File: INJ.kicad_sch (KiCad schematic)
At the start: 10 parts, among them U2 VNLD5160TR-E, U3 VNLD5160TR-E

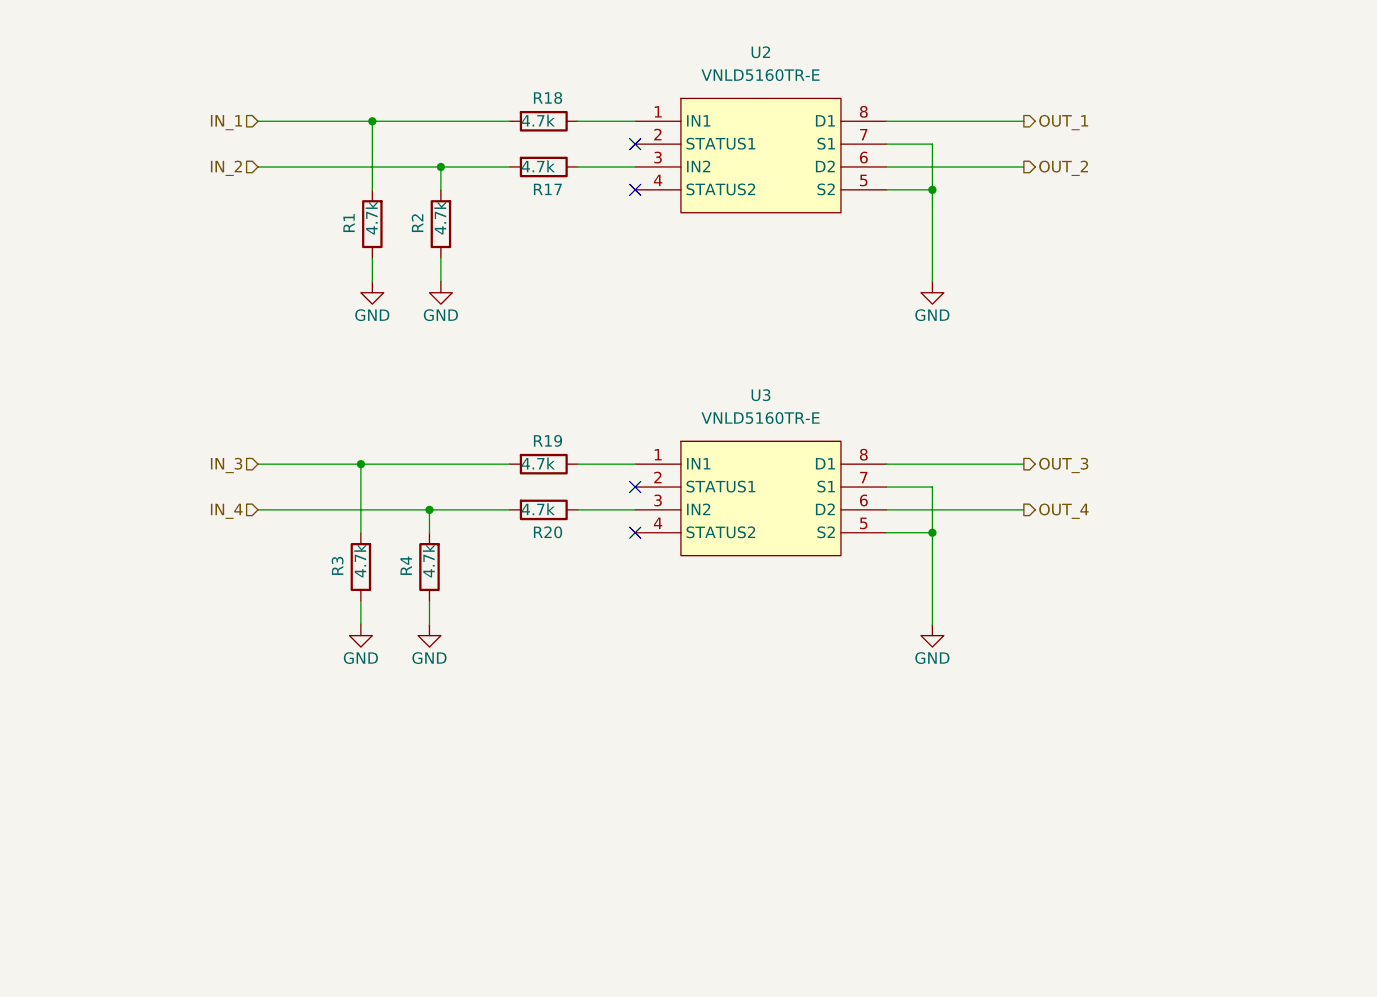
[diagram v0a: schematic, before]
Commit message: Rev D
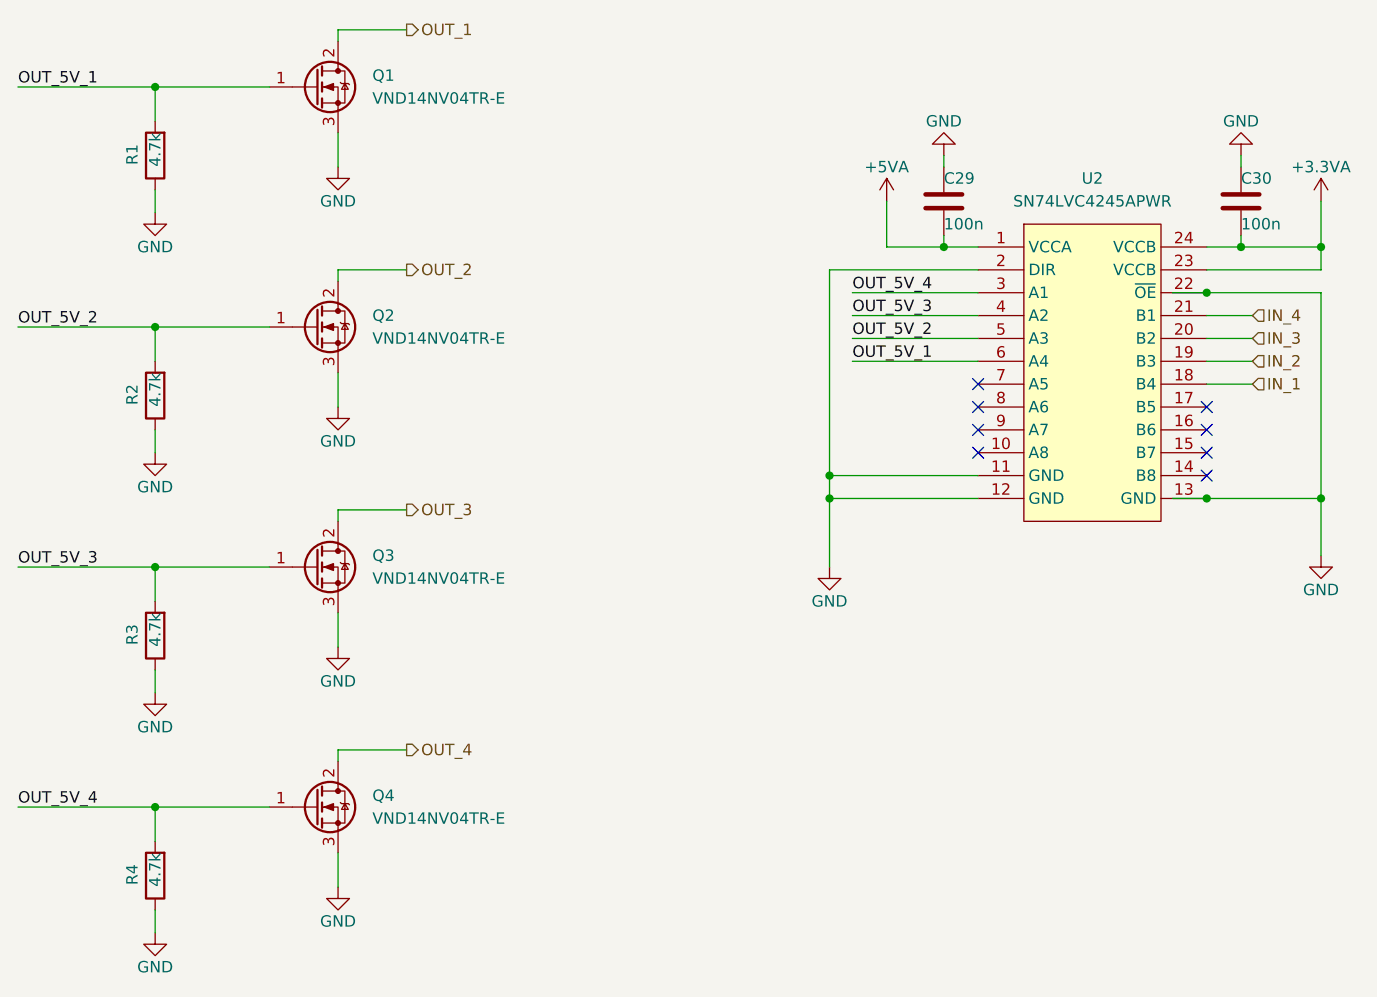
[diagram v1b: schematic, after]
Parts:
- removed R17, R18, R19, R20: 4.7k, Hellen:R0603, symbol Device:R
- removed U2, U3: VNLD5160TR-E, Package_SO:SOIC-8_3.9x4.9mm_P1.27mm, symbol chips:VNLD5160
- added C29, C30: 100n, Capacitor_SMD:C_0603_1608Metric, symbol Device:C
- added Q1, Q2, Q3, Q4: VND14NV04TR-E, Package_TO_SOT_SMD:TO-252-2, symbol semiconductors:VND14NV04TR-E
- added U2: SN74LVC4245APWR, EasyEda2Kicad:TSSOP-24_L7.8-W4.4-P0.65-LS6.4-BL, symbol easyeda2kicad:SN74LVC4245APWR
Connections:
- net GND: now also C29.1, C30.1, Q1.3 (S), Q2.3 (S), Q3.3 (S), Q4.3 (S), U2.11 (GND), U2.12 (GND), U2.13 (GND), U2.2 (DIR), U2.22 (~{OE})
- net IN_1: now also U2.18 (B4); no longer R1.2
- net IN_2: now also U2.19 (B3); no longer R2.2
- net IN_3: now also U2.20 (B2); no longer R3.2
- net IN_4: now also U2.21 (B1); no longer R4.2
- net OUT_1: now also Q1.2 (D)
- net OUT_2: now also Q2.2 (D)
- net OUT_3: now also Q3.2 (D)
- net OUT_4: now also Q4.2 (D)
- new net +3.3VA: C30.2, U2.23 (VCCB), U2.24 (VCCB)
- new net +5VA: C29.2, U2.1 (VCCA)
- new net OUT_5V_1: Q1.1 (G), R1.2, U2.6 (A4)
- new net OUT_5V_2: Q2.1 (G), R2.2, U2.5 (A3)
- new net OUT_5V_3: Q3.1 (G), R3.2, U2.4 (A2)
- new net OUT_5V_4: Q4.1 (G), R4.2, U2.3 (A1)
- no-connect marks 4 -> 8
